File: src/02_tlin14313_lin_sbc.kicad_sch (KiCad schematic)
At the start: 0 parts

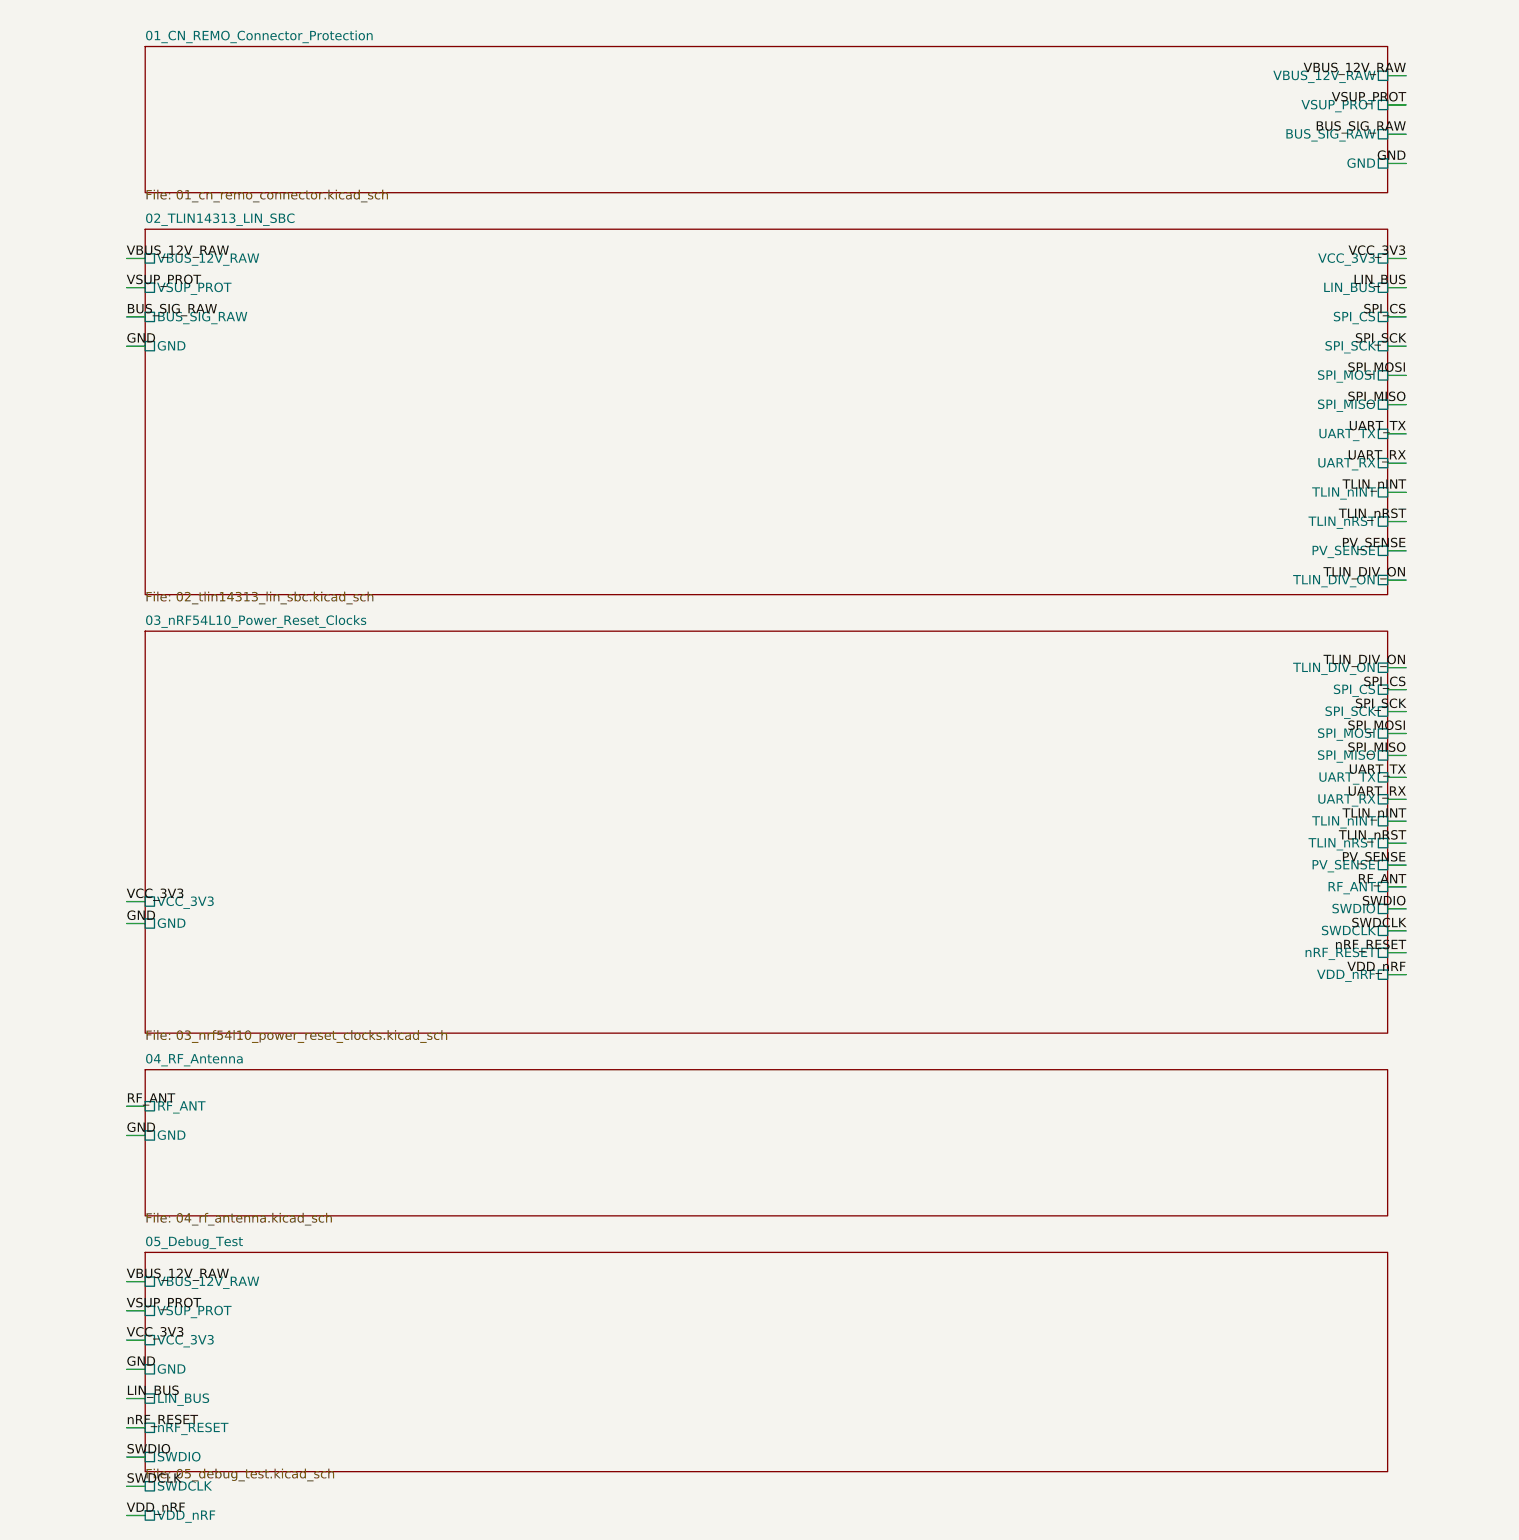
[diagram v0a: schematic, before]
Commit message: stage
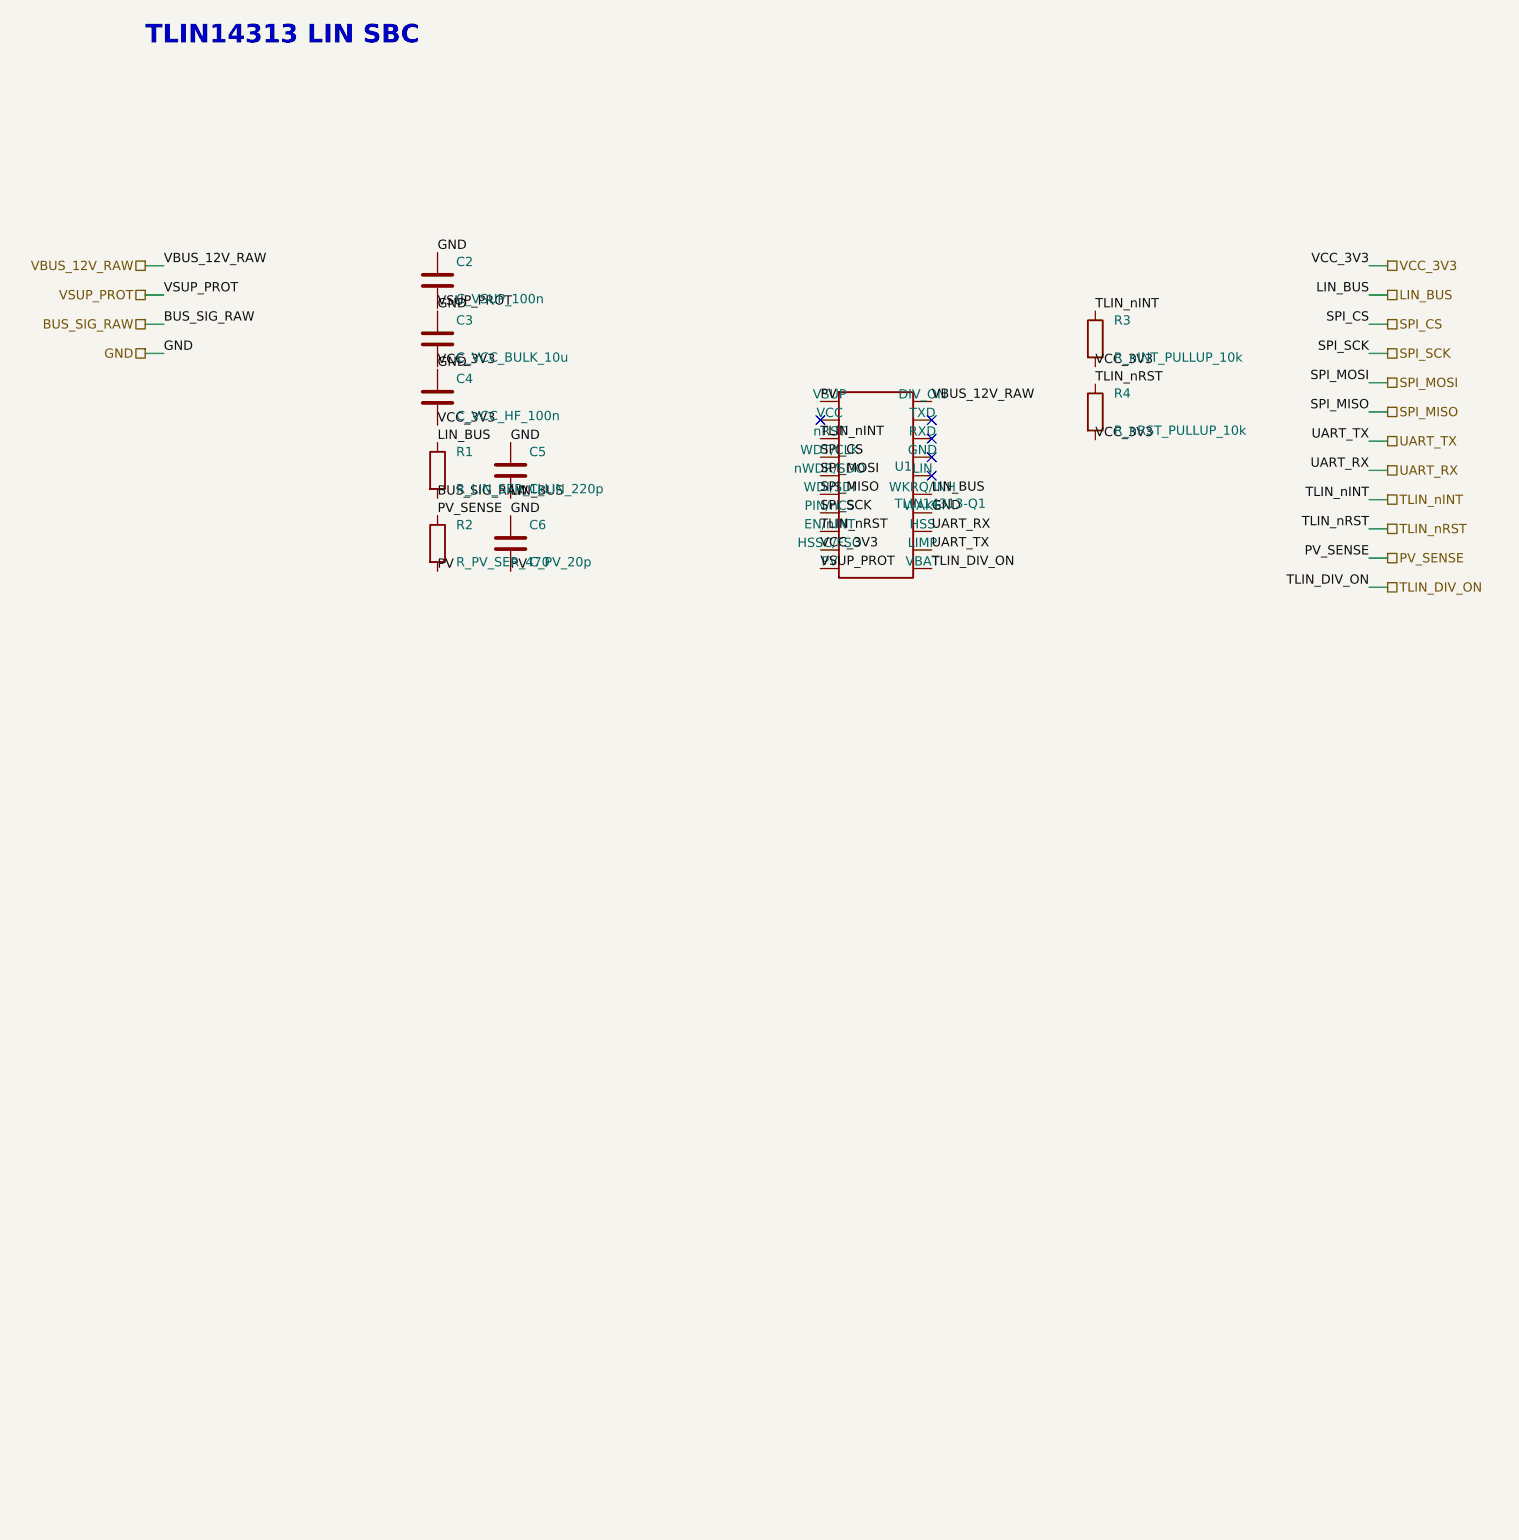
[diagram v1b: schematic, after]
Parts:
- added C2: C_VSUP_100n, symbol Device:C
- added C3: C_VCC_BULK_10u, symbol Device:C
- added C4: C_VCC_HF_100n, symbol Device:C
- added C5: C_LIN_220p, symbol Device:C
- added C6: C_PV_20p, symbol Device:C
- added R1: R_LIN_SER_1k, symbol Device:R
- added R2: R_PV_SER_470, symbol Device:R
- added R3: R_nINT_PULLUP_10k, symbol Device:R
- added R4: R_nRST_PULLUP_10k, symbol Device:R
- added U1: TLIN14313-Q1, symbol HVAC:TLIN14313-Q1
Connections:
- net BUS_SIG_RAW: now also R1.2
- net GND: now also C2.1, C3.1, C4.1, C5.1, C6.1, U1.17 (WAKE)
- net LIN_BUS: now also C5.2, R1.1, U1.16 (WKRQ/INH)
- net PV_SENSE: now also R2.1
- net SPI_CS: now also U1.4 (WDT/CLK)
- net SPI_MISO: now also U1.6 (WDI/SDI)
- net SPI_MOSI: now also U1.5 (nWDR/SDO)
- net SPI_SCK: now also U1.7 (PIN/nCS)
- net TLIN_DIV_ON: now also U1.20 (VBAT)
- net TLIN_nINT: now also R3.1, U1.3 (nRST)
- net TLIN_nRST: now also R4.1, U1.8 (EN/nINT)
- net UART_RX: now also U1.18 (HSS)
- net UART_TX: now also U1.19 (LIMP)
- net VBUS_12V_RAW: now also U1.11 (DIV_ON)
- net VCC_3V3: now also C3.2, C4.2, R3.2, R4.2, U1.9 (HSSC/FSO)
- net VSUP_PROT: now also C2.2, U1.10 (PV)
- new net PV: C6.2, R2.2, U1.1 (VSUP)
- no-connect marks 0 -> 5
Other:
- removed sheet 01_CN_REMO_Connector_Protection
- removed sheet 02_TLIN14313_LIN_SBC
- removed sheet 03_nRF54L10_Power_Reset_Clocks
- removed sheet 04_RF_Antenna
- removed sheet 05_Debug_Test
- note added: "TLIN14313 LIN SBC"
